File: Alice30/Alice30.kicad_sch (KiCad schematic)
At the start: 79 parts, among them J1 USB_B_Mini, SW1 SW_Push_45deg, SW10 SW_Push_45deg, SW11 SW_Push_45deg, SW12 SW_Push_45deg, SW13 SW_Push_45deg, SW14 SW_Push_45deg, SW15 SW_Push_45deg, SW16 SW_Push_45deg, SW17 SW_Push_45deg, SW18 SW_Push_45deg, SW19 SW_Push_45deg, SW2 SW_Push_45deg, SW20 SW_Push_45deg, SW21 SW_Push_45deg, SW22 SW_Push_45deg, SW23 SW_Push_45deg, SW24 SW_Push_45deg, SW25 SW_Push_45deg, SW26 SW_Push_45deg, SW27 SW_Push_45deg, SW28 SW_Push_45deg, SW29 SW_Push_45deg, SW3 SW_Push_45deg, SW30 SW_Push_45deg, SW31 SW_Push_45deg, SW32 SW_Push_45deg, SW33 SW_Push_45deg, SW34 SW_Push_45deg, SW38 SW_Push, SW4 SW_Push_45deg, SW5 SW_Push_45deg, SW6 SW_Push_45deg, SW7 SW_Push_45deg, SW8 SW_Push_45deg, SW9 SW_Push_45deg, U1 ATmega32U2-A, Y1 Crystal_GND24_Small

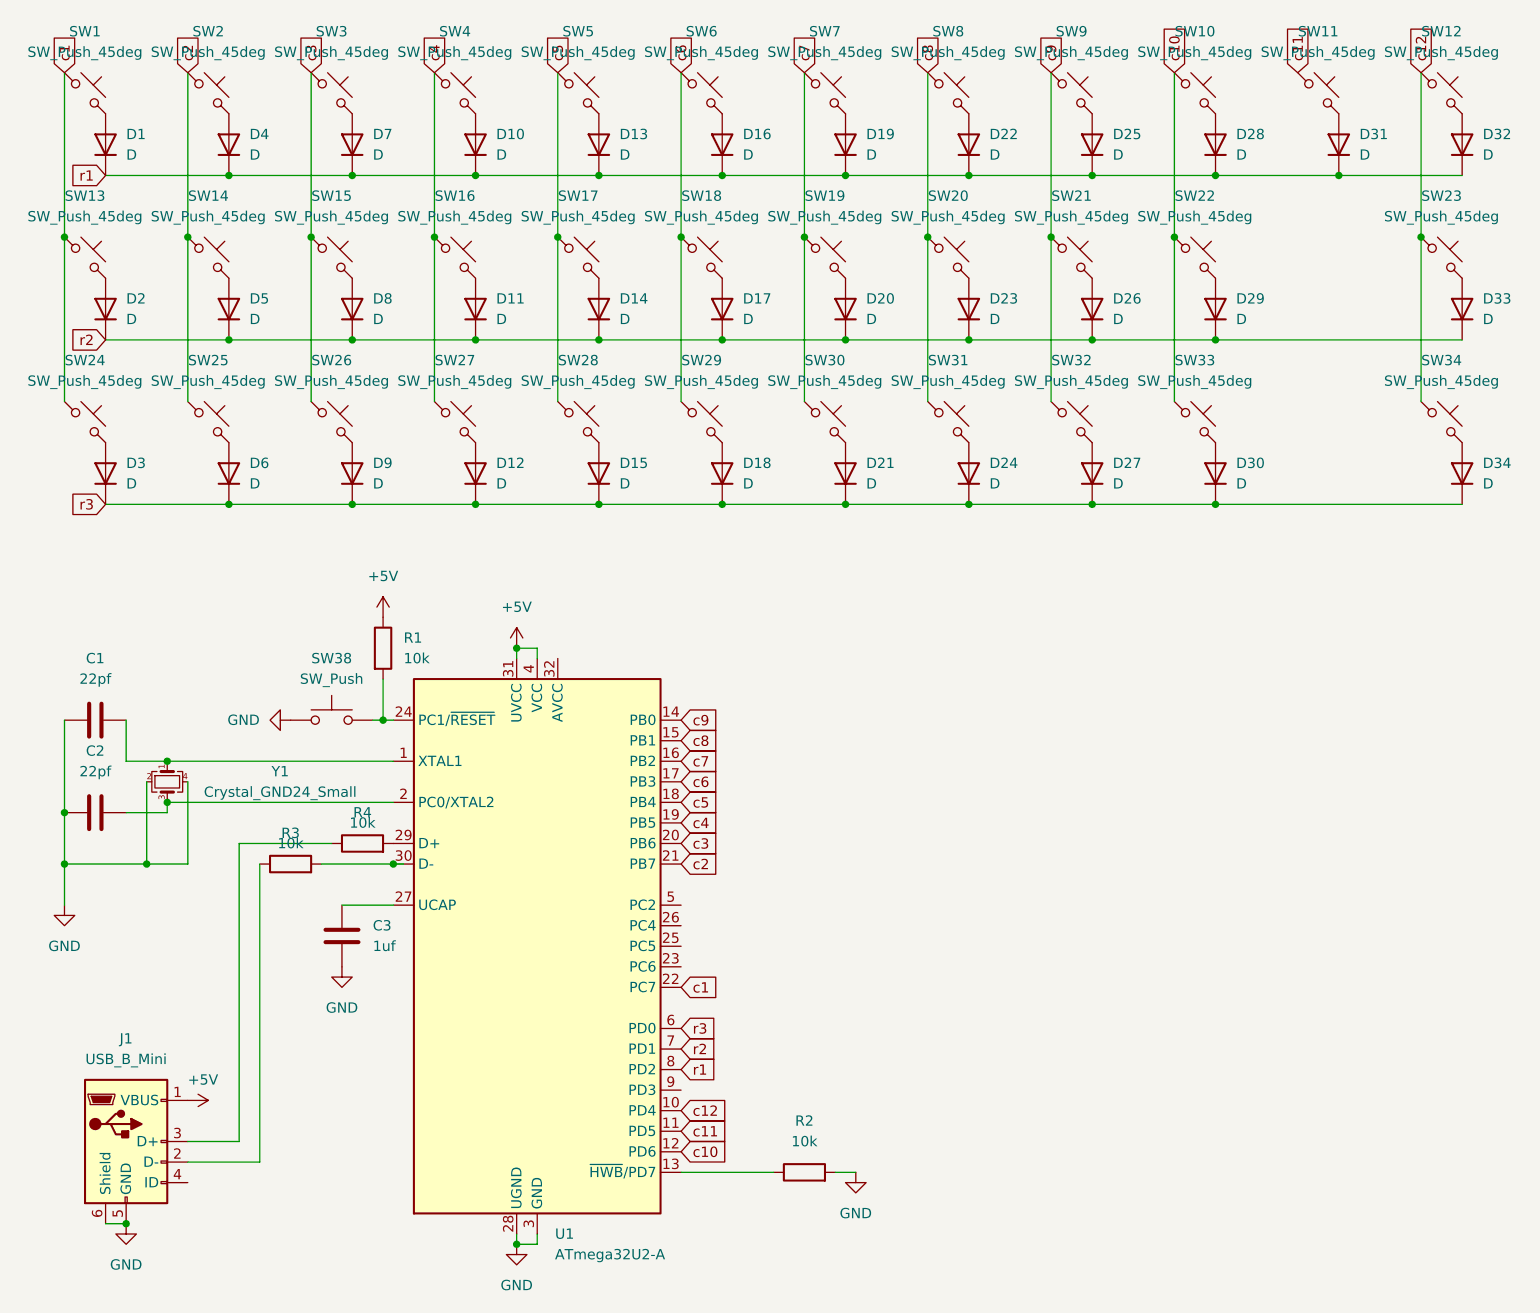
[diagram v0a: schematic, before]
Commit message: .
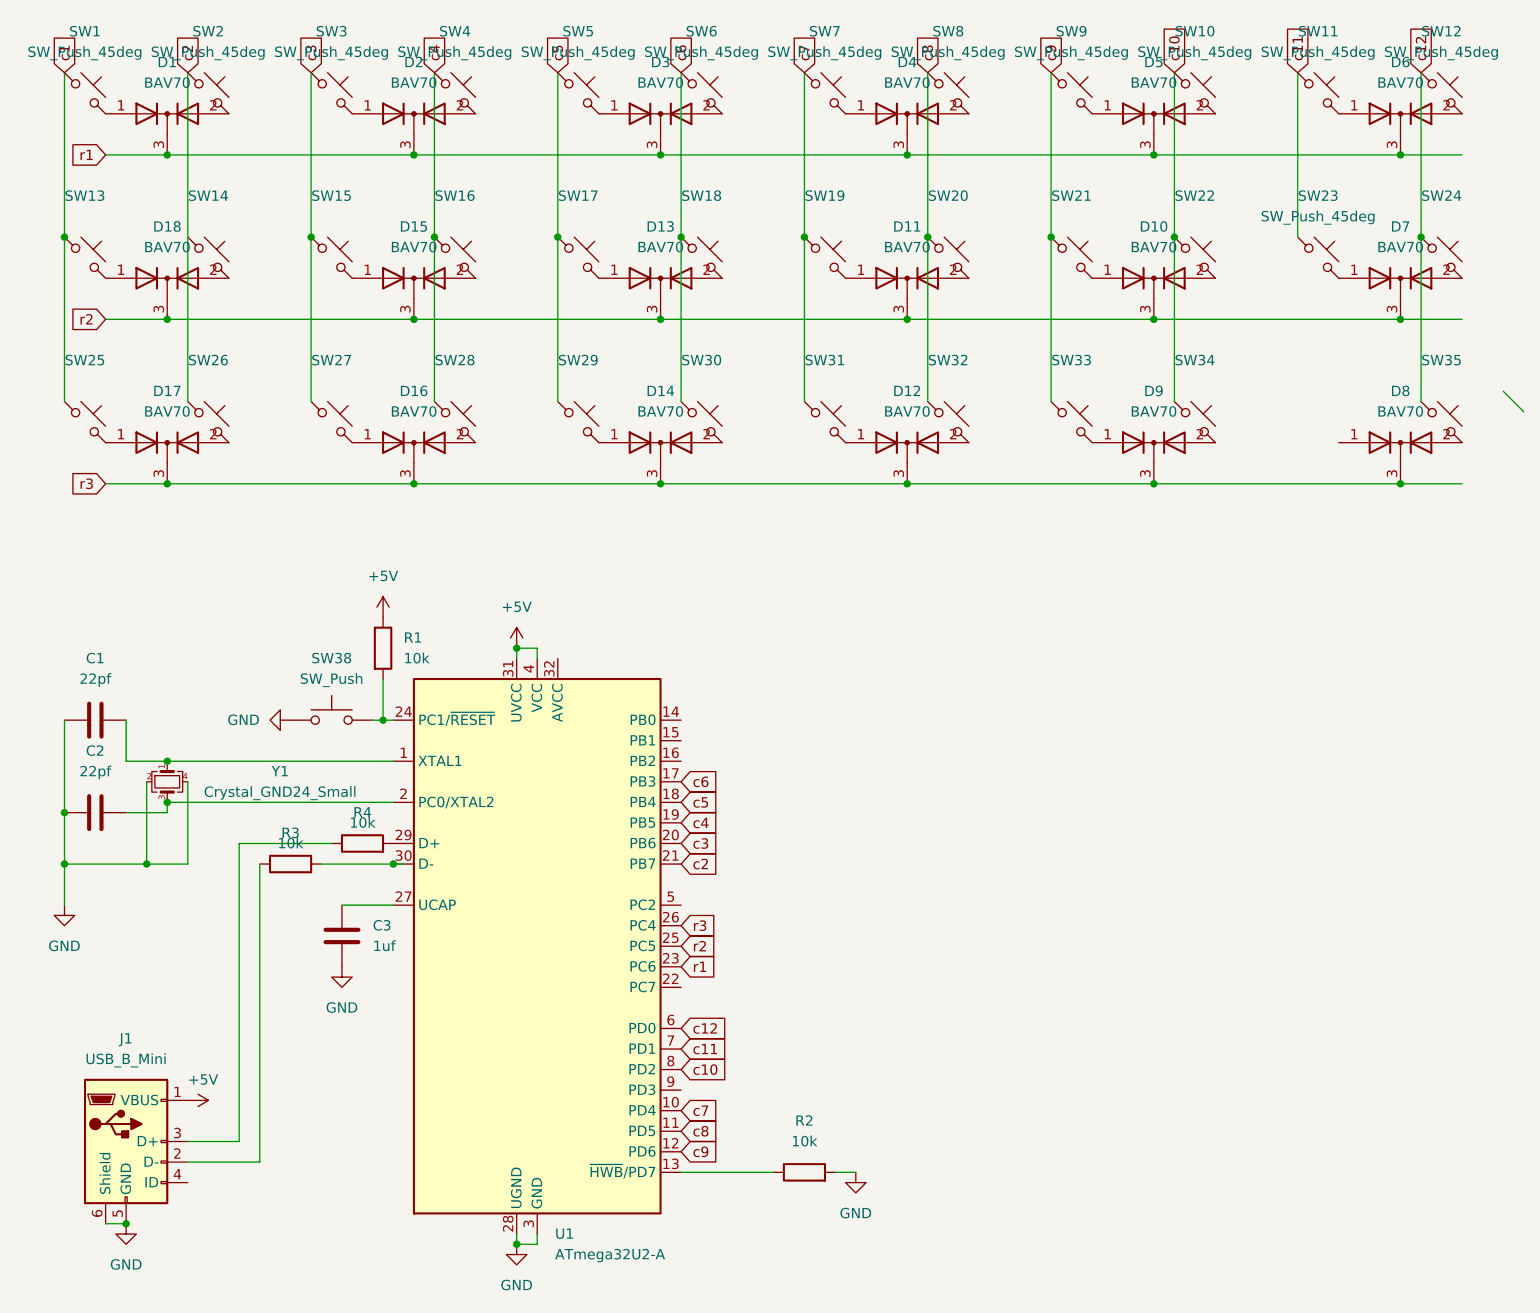
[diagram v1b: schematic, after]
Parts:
- removed D1, D10, D11, D12, D13, D14, D15, D16, D17, D18, D19, D2, D20, D21, D22, D23, D24, D25, D26, D27, D28, D29, D3, D30, D31, D32, D33, D34, D4, D5, D6, D7, D8, D9: D, custom-parts:D_TH, symbol Device:D
- added D1, D10, D11, D12, D13, D14, D15, D16, D17, D18, D2, D3, D4, D5, D6, D7, D8, D9: BAV70, Package_TO_SOT_SMD:SOT-23, symbol Diode:BAV70
- added SW23: SW_Push_45deg, custom-parts:MX_1U_Plate, symbol Switch:SW_Push_45deg
- SW1, SW10, SW11, SW12, SW14, SW15, SW16, SW17, SW18, SW19, SW2, SW20, SW21, SW22, SW3, SW4, SW5, SW6, SW7, SW8, SW9: footprint custom-parts:MX_1U -> custom-parts:MX_1U_Plate
- SW13: footprint custom-parts:MX_1.25U -> custom-parts:MX_1U_Plate
- SW24: renamed from SW23; footprint custom-parts:MX_1.75U -> custom-parts:MX_1U_Plate
- SW25: renamed from SW24; footprint custom-parts:MX_1.25U -> custom-parts:MX_1U_Plate
- SW26: renamed from SW25; footprint custom-parts:MX_1U -> custom-parts:MX_1U_Plate
- SW27: renamed from SW26; footprint custom-parts:MX_1U -> custom-parts:MX_1U_Plate
- SW28: renamed from SW27; footprint custom-parts:MX_1U -> custom-parts:MX_1U_Plate
- SW29: renamed from SW28; footprint custom-parts:MX_1U -> custom-parts:MX_1U_Plate
- SW30: renamed from SW29; footprint custom-parts:MX_1U -> custom-parts:MX_1U_Plate
- SW31: renamed from SW30; footprint custom-parts:MX_1.5U -> custom-parts:MX_1U_Plate
- SW32: renamed from SW31; footprint custom-parts:MX_1U -> custom-parts:MX_1U_Plate
- SW33: renamed from SW32; footprint custom-parts:MX_1U -> custom-parts:MX_1U_Plate
- SW34: renamed from SW33; footprint custom-parts:MX_1U -> custom-parts:MX_1U_Plate
- SW35: renamed from SW34; footprint custom-parts:MX_1.25U -> custom-parts:MX_1U_Plate
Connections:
- net c1: no longer U1.22 (PC7)
- net c10: now also U1.8 (PD2); no longer U1.12 (PD6)
- net c11: now also U1.7 (PD1), SW23.1; no longer U1.11 (PD5)
- net c12: now also U1.6 (PD0); no longer U1.10 (PD4)
- net c2: no longer SW14.1
- net c7: now also U1.10 (PD4); no longer U1.16 (PB2)
- net c8: now also U1.11 (PD5); no longer U1.15 (PB1)
- net c9: now also U1.12 (PD6); no longer U1.14 (PB0)
- net r1: now also U1.23 (PC6), D1.3 (K), D2.3 (K), D3.3 (K), D4.3 (K), D5.3 (K), D6.3 (K); no longer U1.8 (PD2)
- net r2: now also U1.25 (PC5), D10.3 (K), D11.3 (K), D13.3 (K), D15.3 (K), D18.3 (K), D7.3 (K); no longer U1.7 (PD1)
- net r3: now also U1.26 (PC4), D12.3 (K), D14.3 (K), D16.3 (K), D17.3 (K), D8.3 (K), D9.3 (K); no longer U1.6 (PD0)
- net at SW16.2: now also D15.2 (A)
- net at SW10.2: now also D5.2 (A)
- net at SW15.2: now also D15.1 (A)
- net at SW26.2: now also D17.2 (A)
- net at SW27.2: now also D16.1 (A)
- net at SW18.2: now also D13.2 (A)
- net at SW9.2: now also D5.1 (A)
- net at SW12.2: now also D6.2 (A)
- net at SW5.2: now also D3.1 (A)
- net at SW20.2: now also D11.2 (A)
- net at SW22.2: now also D10.2 (A)
- net at SW31.2: now also D12.1 (A)
- net at SW24.2: now also D7.2 (A)
- net at SW14.2: now also D18.2 (A)
- net at SW3.2: now also D2.1 (A)
- net at SW32.2: now also D12.2 (A)
- net at SW8.2: now also D4.2 (A)
- net at SW28.2: now also D16.2 (A)
- net at SW34.2: now also D9.2 (A)
- net at SW17.2: now also D13.1 (A)
- net at SW6.2: now also D3.2 (A)
- net at SW13.2: now also D18.1 (A)
- net at SW11.2: now also D6.1 (A)
- net at SW30.2: now also D14.2 (A)
- net at SW33.2: now also D9.1 (A)
- net at SW2.2: now also D1.2 (A)
- net at SW19.2: now also D11.1 (A)
- net at SW21.2: now also D10.1 (A)
- net at SW1.2: now also D1.1 (A)
- net at SW29.2: now also D14.1 (A)
- net at SW7.2: now also D4.1 (A)
- net at SW25.2: now also D17.1 (A)
- net at SW4.2: now also D2.2 (A)
- net at SW35.2: now also D8.2 (A)
- new net: D7.1 (A), SW23.2
